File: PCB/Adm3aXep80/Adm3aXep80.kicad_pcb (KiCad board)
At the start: 2 copper layers, 10.3 x 1.7 mm, 10 parts, among them J1 Conn_Coaxial, J2 Conn_01x09, J22 Conn_01x13, J8 Conn_01x13

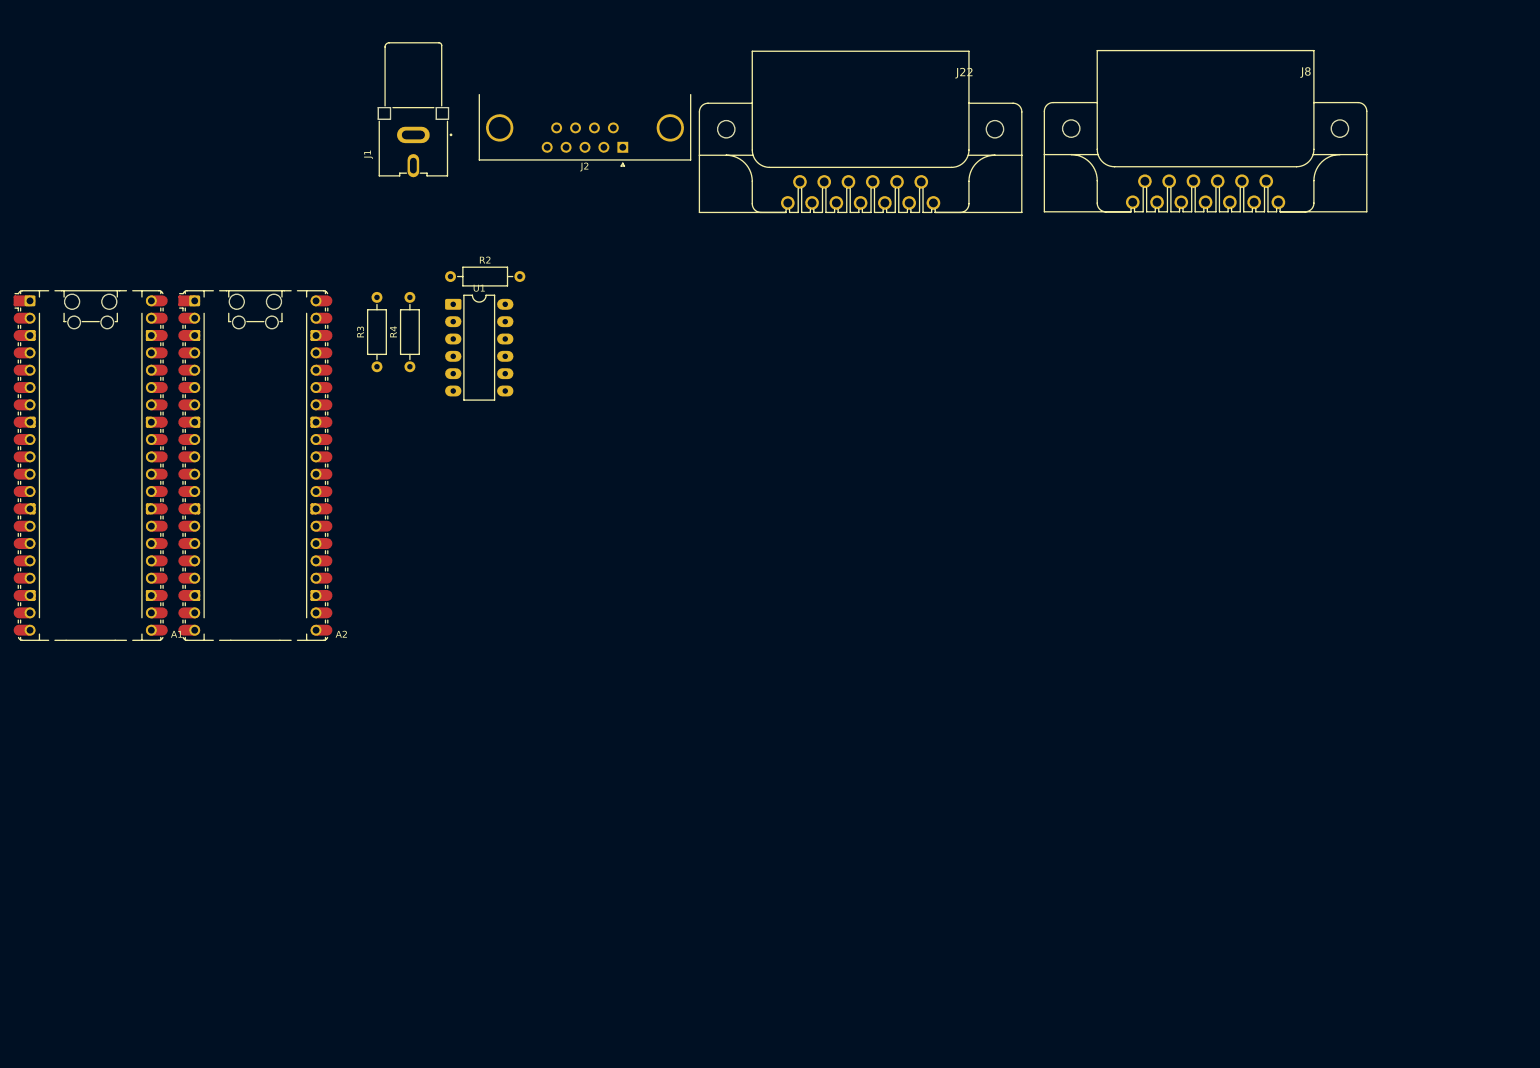
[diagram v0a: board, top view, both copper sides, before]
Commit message: PCB
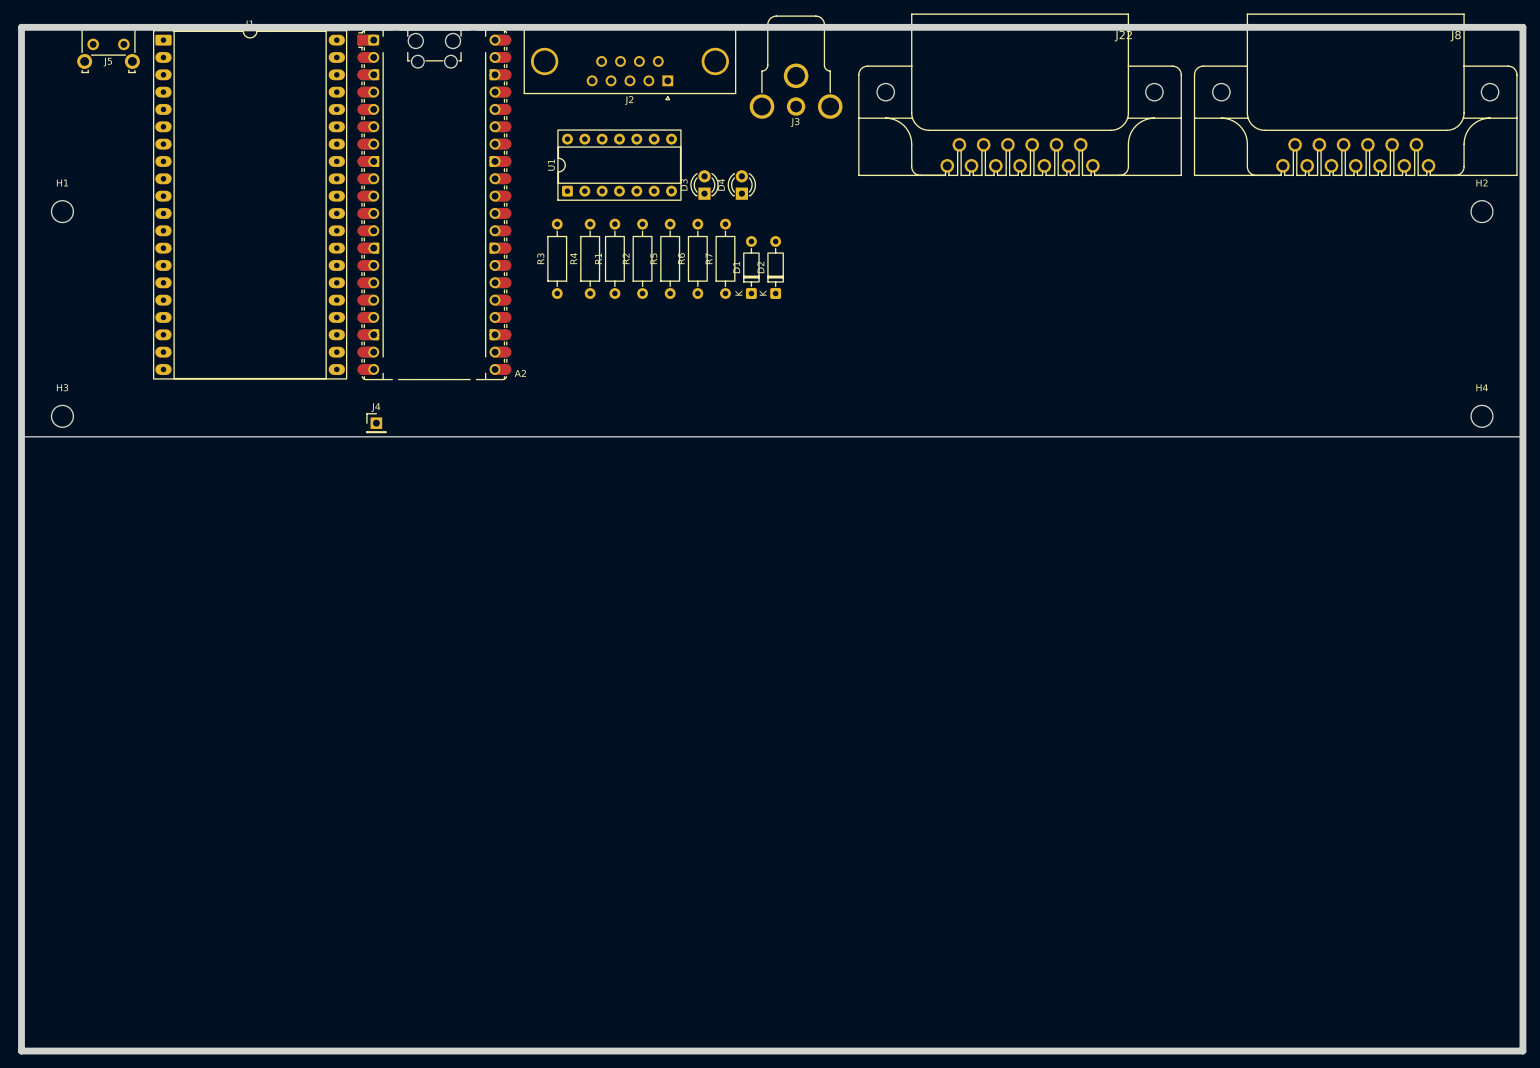
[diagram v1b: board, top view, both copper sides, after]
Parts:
- removed A1: RaspberryPi_Pico, Module:RaspberryPi_Pico_Common_Unspecified
- added D1: 1N4148, Diode_THT:D_DO-35_SOD27_P7.62mm_Horizontal, F.Cu at (171.4, 51.5)
- added D2: 1N4148, Diode_THT:D_DO-35_SOD27_P7.62mm_Horizontal, F.Cu at (175.0, 51.5)
- added D3: LED, LED_THT:LED_D3.0mm, F.Cu at (164.6, 36.9)
- added D4: LED, LED_THT:LED_D3.0mm, F.Cu at (170.1, 36.9)
- added H1: MountingHole, MountingHole:MountingHole_3.2mm_M3, F.Cu at (70.5, 39.5)
- added H2: MountingHole, MountingHole:MountingHole_3.2mm_M3, F.Cu at (278.5, 39.5)
- added H3: MountingHole, MountingHole:MountingHole_3.2mm_M3, F.Cu at (70.5, 69.5)
- added H4: MountingHole, MountingHole:MountingHole_3.2mm_M3, F.Cu at (278.5, 69.5)
- added J3: Conn_Coaxial, RCA:RCA-Phono_CUI-Devices_RCJ-01X_Horizontal, F.Cu at (178.0, 24.1)
- added J4: prog, Connector_PinHeader_2.54mm:PinHeader_1x01_P2.54mm_Vertical, F.Cu at (116.5, 70.5)
- added J5: Conn_01x04, Button_Switch_THT:SW_Tactile_SKHH_Angled, F.Cu at (75.0, 15.0)
- added R1: 1K, Resistor_THT:R_Axial_DIN0207_L6.3mm_D2.5mm_P10.16mm_Horizontal, F.Cu at (151.4, 51.5)
- added R5: 1K, Resistor_THT:R_Axial_DIN0207_L6.3mm_D2.5mm_P10.16mm_Horizontal, F.Cu at (159.6, 51.5)
- added R6: 1K, Resistor_THT:R_Axial_DIN0207_L6.3mm_D2.5mm_P10.16mm_Horizontal, F.Cu at (163.6, 51.5)
- added R7: 1K, Resistor_THT:R_Axial_DIN0207_L6.3mm_D2.5mm_P10.16mm_Horizontal, F.Cu at (167.7, 51.5)
- J1: value Conn_Coaxial -> HDMI; footprint Atari:CUI_RCJ-043 -> Package_DIP:DIP-40_W25.4mm_Socket_LongPads
- R2: value 1K -> 2.2K
- U1: value ~ -> 74125; footprint Package_DIP:DIP-12_W7.62mm_LongPads -> Package_DIP:DIP-14_W7.62mm_Socket
- moved A2 46.3 mm to (125.0, 38.5)
- moved J1 37.9 mm to (85.3, 14.4), turned to 0 degrees
- moved R3 28.5 mm to (143.0, 51.5)
- moved R4 28.5 mm to (147.8, 51.5)
- moved R2 28.2 mm to (155.5, 51.5), turned to 90 degrees
- moved J22 24.0 mm to (209.5, 22.0)
- moved U1 23.6 mm to (144.5, 36.5), turned to 90 degrees
- moved J8 22.6 mm to (258.7, 22.0)
- moved J2 11.8 mm to (159.2, 20.3)
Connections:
- A2 pad 39: SIORDY -> Net-(A2-VSYS)
- A2 pad 4: unconnected-(A2-GPIO2-Pad4) -> SERIN
- A2 pad 5: SERIN -> SEROUT
- A2 pad 6: SEROUT -> JOYEN
- A2 pad 7: unconnected-(A2-GPIO5-Pad7) -> JOYEN\
- J1 pad 1: Net-(J1-In) -> unconnected-(J1-Pin_1-Pad1)
- J1 pad 2: GND -> unconnected-(J1-Pin_2-Pad2)
- J2 pad 7: SIORDY -> JOY5V
- R2 pad 2: SIO_Motor -> JOYEN
- R3 pad 1: Net-(J1-In) -> Net-(J3-In)
- R4 pad 1: Net-(J1-In) -> Net-(J3-In)
- U1 pad 1: SERIN -> JOYEN
- U1 pad 10: SIORDY -> JOYEN
- U1 pad 11: SIO_Proceed -> SERIN
- U1 pad 12: SIO_Motor -> JOY1
- U1 pad 3: +3V3 -> SIO_Proceed
- U1 pad 4: GND -> JOYEN\
- U1 pad 5: SERIN -> SEROUT
- U1 pad 6: SEROUT -> JOY2
- U1 pad 7: JOY2 -> GND
- U1 pad 8: JOY1 -> SERIN
- U1 pad 9: GND -> SIO_Motor
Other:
- board size 10.3 x 1.7 mm -> 220 x 150 mm
